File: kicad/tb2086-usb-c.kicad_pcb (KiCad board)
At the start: 2 copper layers, 29.3 x 19.5 mm, 17 parts, among them J1 Conn_01x04, U1 USBLC6-2SC6

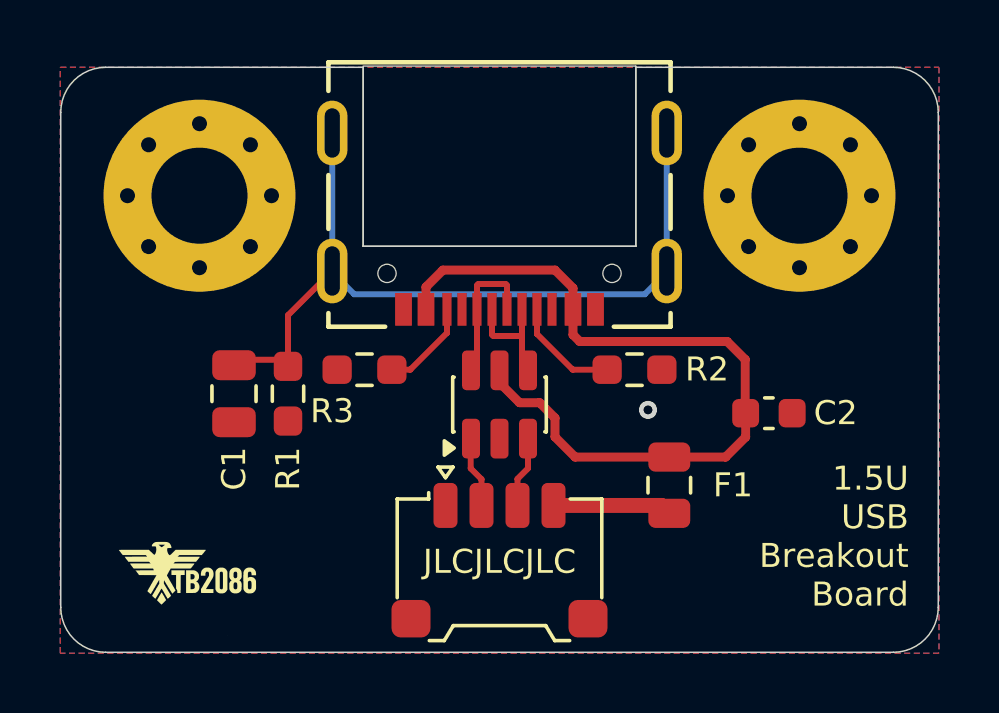
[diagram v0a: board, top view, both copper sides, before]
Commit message: changed footprint (#7)
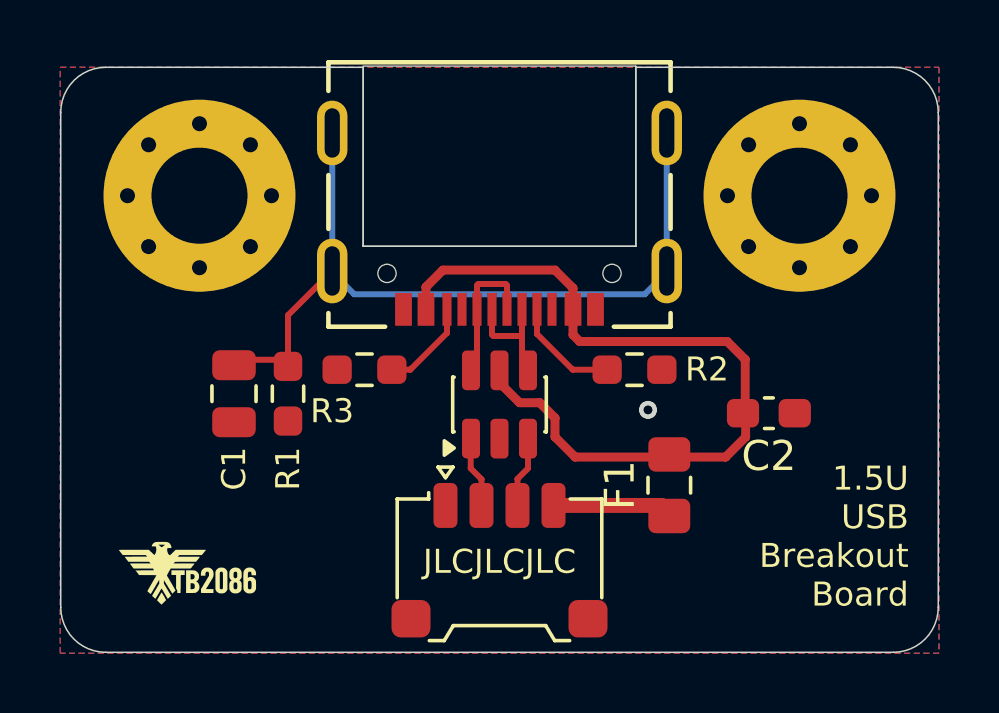
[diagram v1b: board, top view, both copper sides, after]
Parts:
- C2: footprint Capacitor_SMD:C_0603_1608Metric -> Capacitor_SMD:C_0603_1608Metric_Pad1.08x0.95mm_HandSolder
- F1: footprint Fuse:Fuse_0805_2012Metric -> Fuse:Fuse_0805_2012Metric_Pad1.15x1.40mm_HandSolder
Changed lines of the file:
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@@
 		(embedded_fonts no)
 	)
-	(footprint "Fuse:Fuse_0805_2012Metric"
+	(footprint "Fuse:Fuse_0805_2012Metric_Pad1.15x1.40mm_HandSolder"
 		(layer "F.Cu")
 		(at 122.21 72.43 90)
-		(descr "Fuse SMD 0805 (2012 Metric), square (rectangular) end terminal, IPC-7351 nominal, (Body size source: https://docs.google.com/spreadsheets/d/1BsfQQcO9C6DZCsRaXUlFlo91Tg2WpOkGARC1WS5S8t0/edit?usp=sharing), generated with kicad-footprint-generator")
-		(tags "fuse")
+		(descr "Fuse SMD 0805 (2012 Metric), square (rectangular) end terminal, IPC-7351 nominal with elongated pad for handsoldering. (Body size source: https://docs.google.com/spreadsheets/d/1BsfQQcO9C6DZCsRaXUlFlo91Tg2WpOkGARC1WS5S8t0/edit?usp=sharing), generated with kicad-footprint-generator")
+		(tags "fuse handsolder")
 		(property "Reference" "F1"
-			(at 0 2.12 0)
-			(layer "F.SilkS")
-			(effects
-				(font
-					(size 0.8 0.8)
+			(at 0 -1.65 90)
+			(layer "F.SilkS")
+			(effects
+				(font
+					(size 1 1)
 					(thickness 0.15)
 				)
@@
 		(attr smd)
 		(fp_line
-			(start -0.258578 -0.71)
-			(end 0.258578 -0.71)
+			(start -0.261252 -0.71)
+			(end 0.261252 -0.71)
 			(stroke
 				(width 0.12)
@@
 		)
 		(fp_line
-			(start -0.258578 0.71)
-			(end 0.258578 0.71)
+			(start -0.261252 0.71)
+			(end 0.261252 0.71)
 			(stroke
 				(width 0.12)
@@
 		)
 		(fp_line
-			(start 1.68 -0.95)
-			(end 1.68 0.95)
+			(start 1.85 -0.95)
+			(end 1.85 0.95)
 			(stroke
 				(width 0.05)
@@
 		)
 		(fp_line
-			(start -1.68 -0.95)
-			(end 1.68 -0.95)
+			(start -1.85 -0.95)
+			(end 1.85 -0.95)
 			(stroke
 				(width 0.05)
@@
 		)
 		(fp_line
-			(start 1.68 0.95)
-			(end -1.68 0.95)
+			(start 1.85 0.95)
+			(end -1.85 0.95)
 			(stroke
 				(width 0.05)
@@
 		)
 		(fp_line
-			(start -1.68 0.95)
-			(end -1.68 -0.95)
+			(start -1.85 0.95)
+			(end -1.85 -0.95)
 			(stroke
 				(width 0.05)
@@
 		)
 		(pad "1" smd roundrect
-			(at -0.9375 0 90)
-			(size 0.975 1.4)
+			(at -1.025 0 90)
+			(size 1.15 1.4)
 			(layers "F.Cu" "F.Mask" "F.Paste")
-			(roundrect_rratio 0.25)
+			(roundrect_rratio 0.217391)
 			(net 10 "+5V")
 			(pintype "passive")
 		)
 		(pad "2" smd roundrect
-			(at 0.9375 0 90)
-			(size 0.975 1.4)
+			(at 1.025 0 90)
+			(size 1.15 1.4)
 			(layers "F.Cu" "F.Mask" "F.Paste")
-			(roundrect_rratio 0.25)
+			(roundrect_rratio 0.217391)
 			(net 2 "VBUS")
 			(pintype "passive")
@@
 		(embedded_fonts no)
 	)
-	(footprint "Capacitor_SMD:C_0603_1608Metric"
+	(footprint "Capacitor_SMD:C_0603_1608Metric_Pad1.08x0.95mm_HandSolder"
 		(layer "F.Cu")
 		(at 125.53 70.03 180)
-		(descr "Capacitor SMD 0603 (1608 Metric), square (rectangular) end terminal, IPC-7351 nominal, (Body size source: IPC-SM-782 page 76, https://www.pcb-3d.com/wordpress/wp-content/uploads/ipc-sm-782a_amendment_1_and_2.pdf), generated with kicad-footprint-generator")
-		(tags "capacitor")
+		(descr "Capacitor SMD 0603 (1608 Metric), square (rectangular) end terminal, IPC-7351 nominal with elongated pad for handsoldering. (Body size source: IPC-SM-782 page 76, https://www.pcb-3d.com/wordpress/wp-content/uploads/ipc-sm-782a_amendment_1_and_2.pdf), generated with kicad-footprint-generator")
+		(tags "capacitor handsolder")
 		(property "Reference" "C2"
-			(at -2.223842 0.006328 0)
-			(layer "F.SilkS")
-			(effects
-				(font
-					(size 0.8 0.8)
+			(at 0 -1.43 180)
+			(layer "F.SilkS")
+			(effects
+				(font
+					(size 1 1)
 					(thickness 0.15)
 				)
@@
 		)
 		(property "Value" "10u"
-			(at 0 1.43 0)
+			(at 0 1.43 180)
 			(layer "F.Fab")
 			(effects
@@
 		)
 		(property "Datasheet" "~"
-			(at 0 0 0)
+			(at 0 0 180)
 			(layer "F.Fab")
 			(hide yes)
@@
 		)
 		(property "Description" ""
-			(at 0 0 0)
+			(at 0 0 180)
 			(layer "F.Fab")
 			(hide yes)
@@
 		(attr smd)
 		(fp_line
-			(start -0.14058 0.51)
-			(end 0.14058 0.51)
+			(start -0.146267 0.51)
+			(end 0.146267 0.51)
 			(stroke
 				(width 0.12)
@@
 		)
 		(fp_line
-			(start -0.14058 -0.51)
-			(end 0.14058 -0.51)
+			(start -0.146267 -0.51)
+			(end 0.146267 -0.51)
 			(stroke
 				(width 0.12)
@@
 		)
 		(fp_line
-			(start 1.48 0.73)
-			(end -1.48 0.73)
+			(start 1.65 0.73)
+			(end -1.65 0.73)
 			(stroke
 				(width 0.05)
@@
 		)
 		(fp_line
-			(start 1.48 -0.73)
-			(end 1.48 0.73)
+			(start 1.65 -0.73)
+			(end 1.65 0.73)
 			(stroke
 				(width 0.05)
@@
 		)
 		(fp_line
-			(start -1.48 0.73)
-			(end -1.48 -0.73)
+			(start -1.65 0.73)
+			(end -1.65 -0.73)
 			(stroke
 				(width 0.05)
@@
 		)
 		(fp_line
-			(start -1.48 -0.73)
-			(end 1.48 -0.73)
+			(start -1.65 -0.73)
+			(end 1.65 -0.73)
 			(stroke
 				(width 0.05)
@@
 		)
 		(fp_text user "${REFERENCE}"
-			(at 0 0 0)
+			(at 0 0 180)
 			(layer "F.Fab")
 			(effects
@@
 		)
 		(pad "1" smd roundrect
-			(at -0.775 0 180)
-			(size 0.9 0.95)
+			(at -0.8625 0 180)
+			(size 1.075 0.95)
 			(layers "F.Cu" "F.Mask" "F.Paste")
 			(roundrect_rratio 0.25)
 			(net 1 "GND")
 			(pintype "passive")
-			(zone_connect 2)
 		)
 		(pad "2" smd roundrect
-			(at 0.775 0 180)
-			(size 0.9 0.95)
+			(at 0.8625 0 180)
+			(size 1.075 0.95)
 			(layers "F.Cu" "F.Mask" "F.Paste")
 			(roundrect_rratio 0.25)
